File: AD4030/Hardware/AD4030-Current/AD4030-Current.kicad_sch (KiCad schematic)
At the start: 0 parts

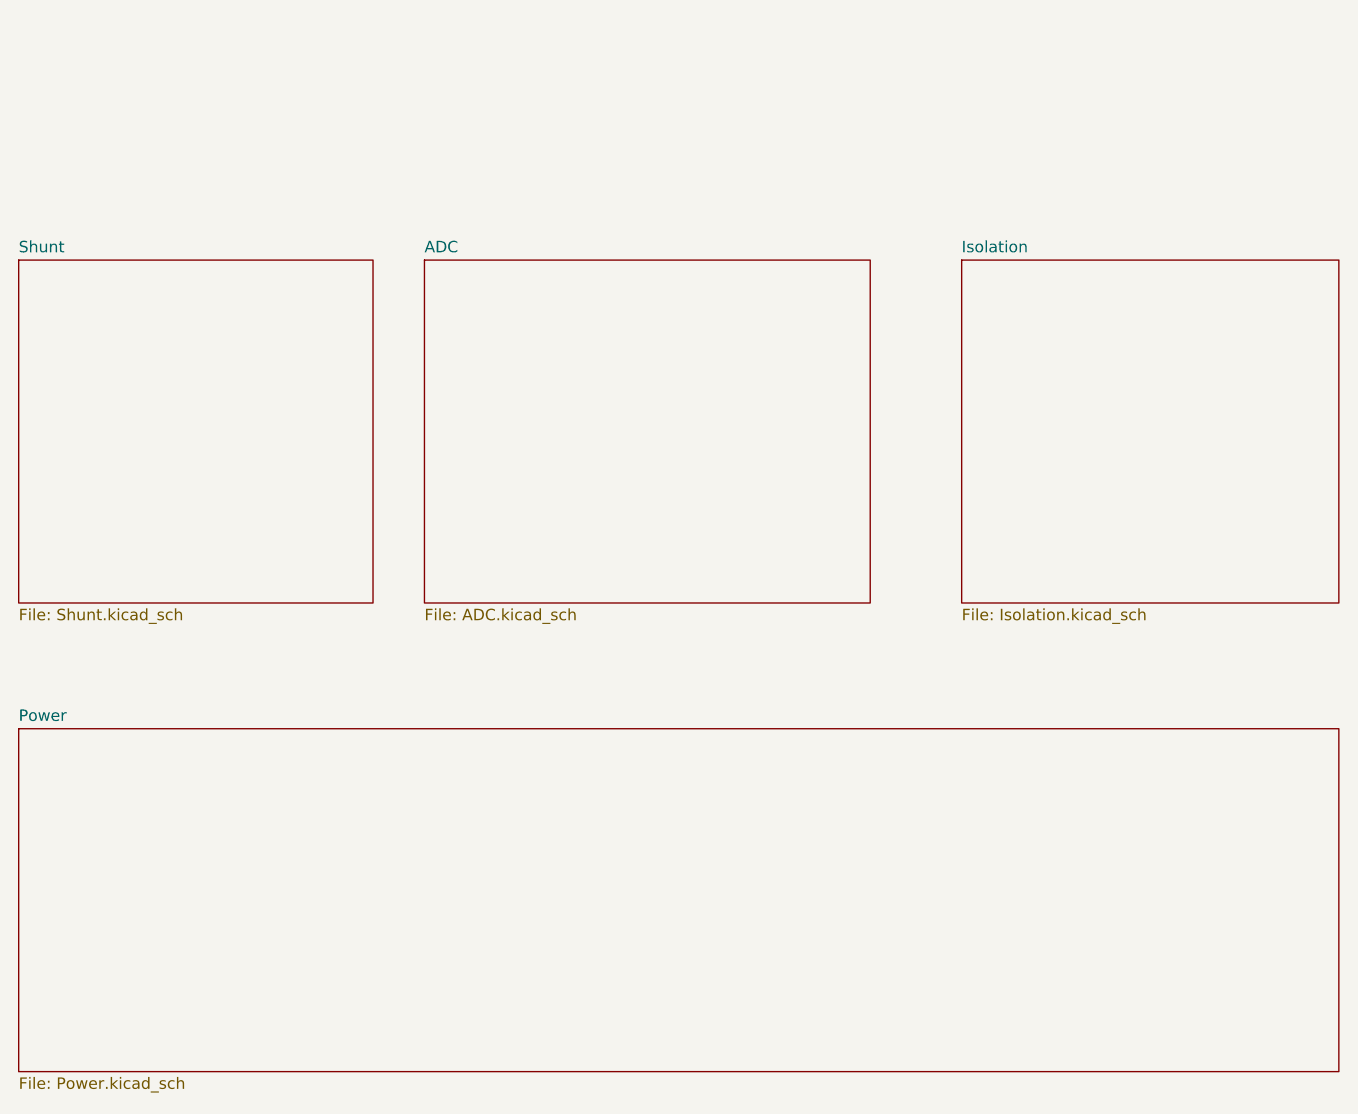
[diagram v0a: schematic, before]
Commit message: Hardware
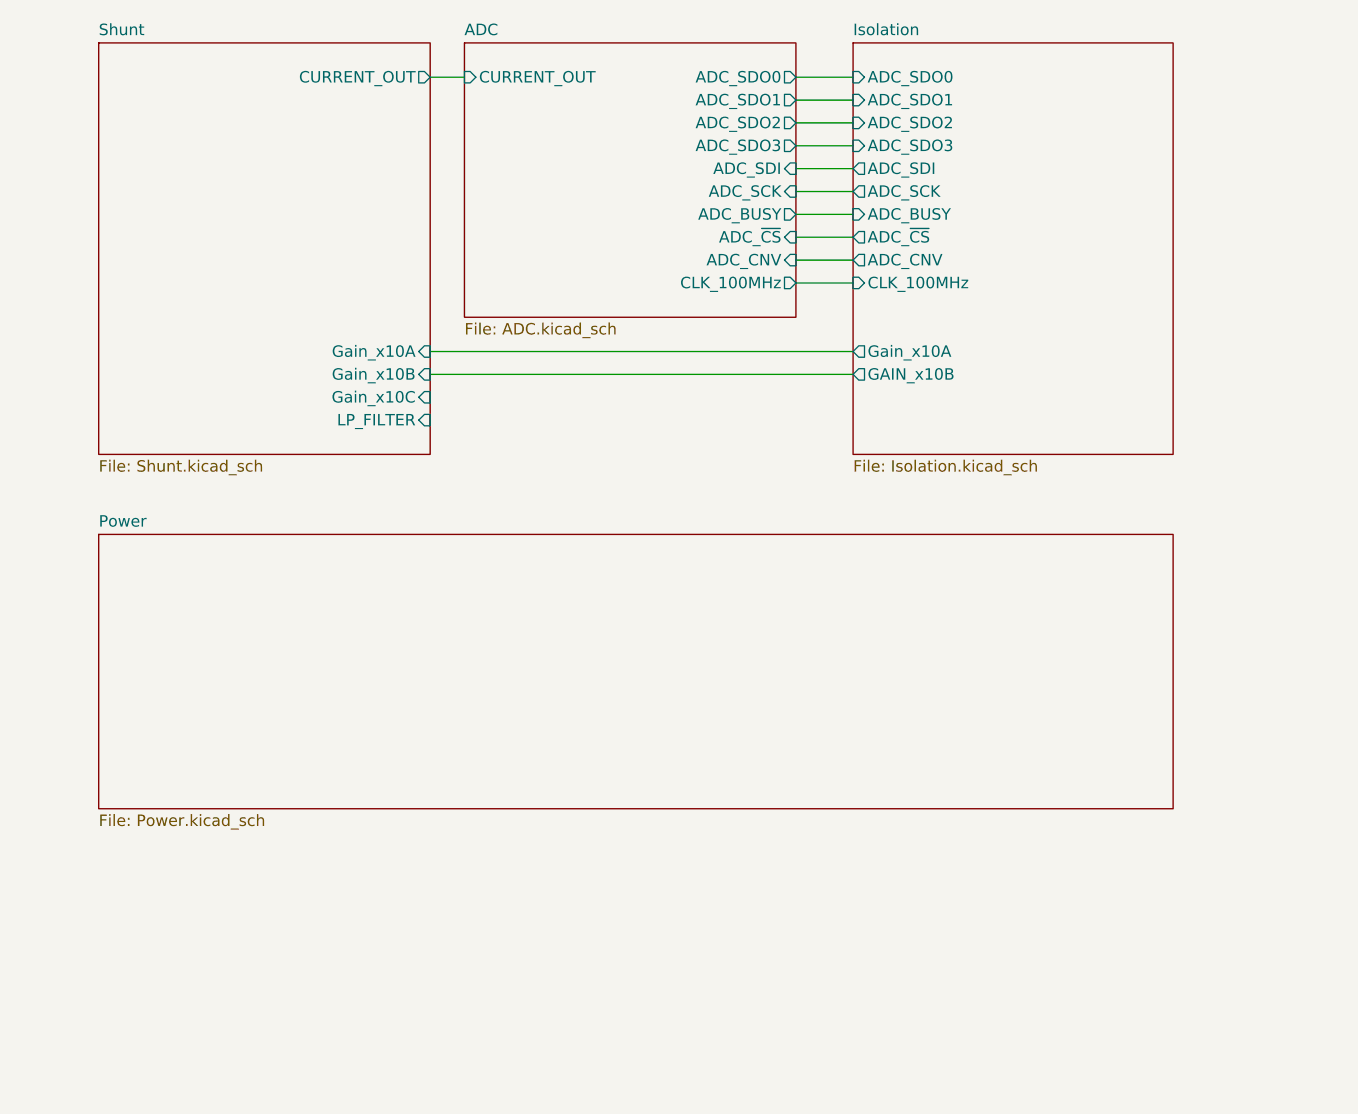
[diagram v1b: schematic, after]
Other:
- sheet ADC ports: added ADC_BUSY, ADC_CNV, ADC_SCK, ADC_SDI, ADC_SDO0, ADC_SDO1, ADC_SDO2, ADC_SDO3, ADC_~{CS}, CLK_100MHz, CURRENT_OUT; removed none
- sheet Isolation ports: added ADC_BUSY, ADC_CNV, ADC_SCK, ADC_SDI, ADC_SDO0, ADC_SDO1, ADC_SDO2, ADC_SDO3, ADC_~{CS}, CLK_100MHz, GAIN_x10B, Gain_x10A; removed none
- sheet Shunt ports: added CURRENT_OUT, Gain_x10A, Gain_x10B, Gain_x10C, LP_FILTER; removed none
